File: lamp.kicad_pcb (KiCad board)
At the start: 4 copper layers, 24 x 24 mm, 47 parts, among them J1 Conn_01x01_Female, J2 Conn_01x01_Female, J3 Conn_01x01_Female, J4 Conn_01x01_Female, J5 Conn_01x01_Female, J6 Conn_01x01_Female, J7 Conn_01x01_Female, U1 STM32F030F4P6, U2 LMV321, U3 MIC5205-3.3, U4 TPS54620, U5 LMV321

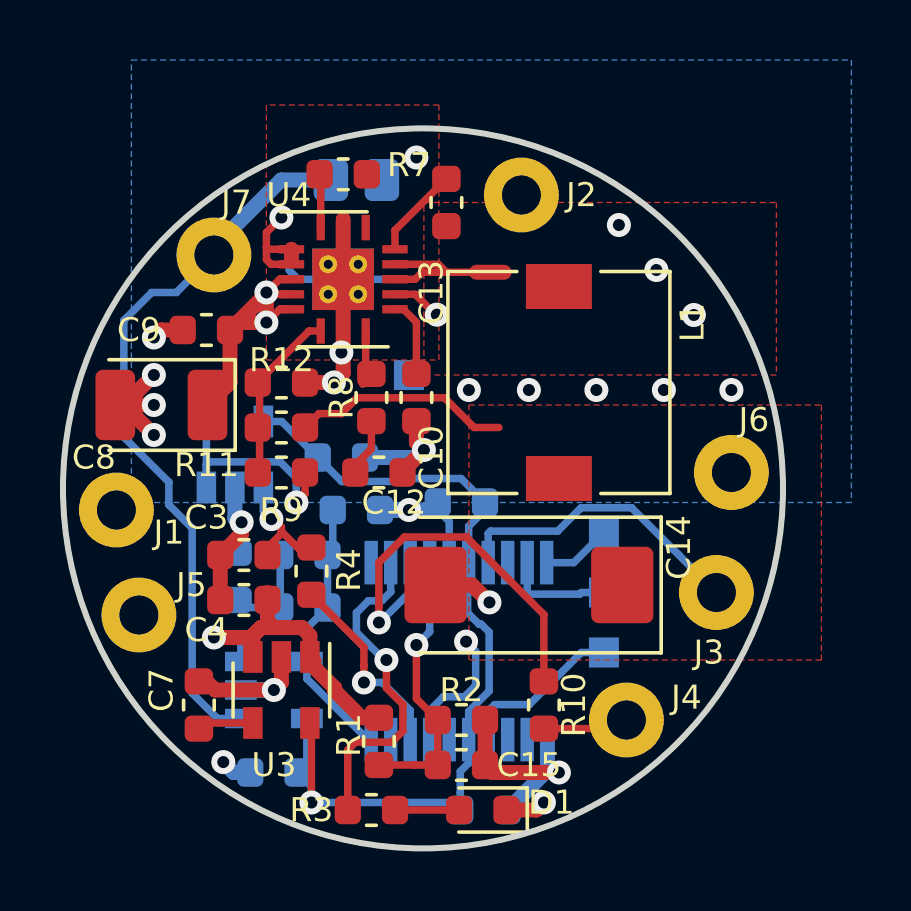
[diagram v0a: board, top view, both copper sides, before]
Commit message: Wibbles
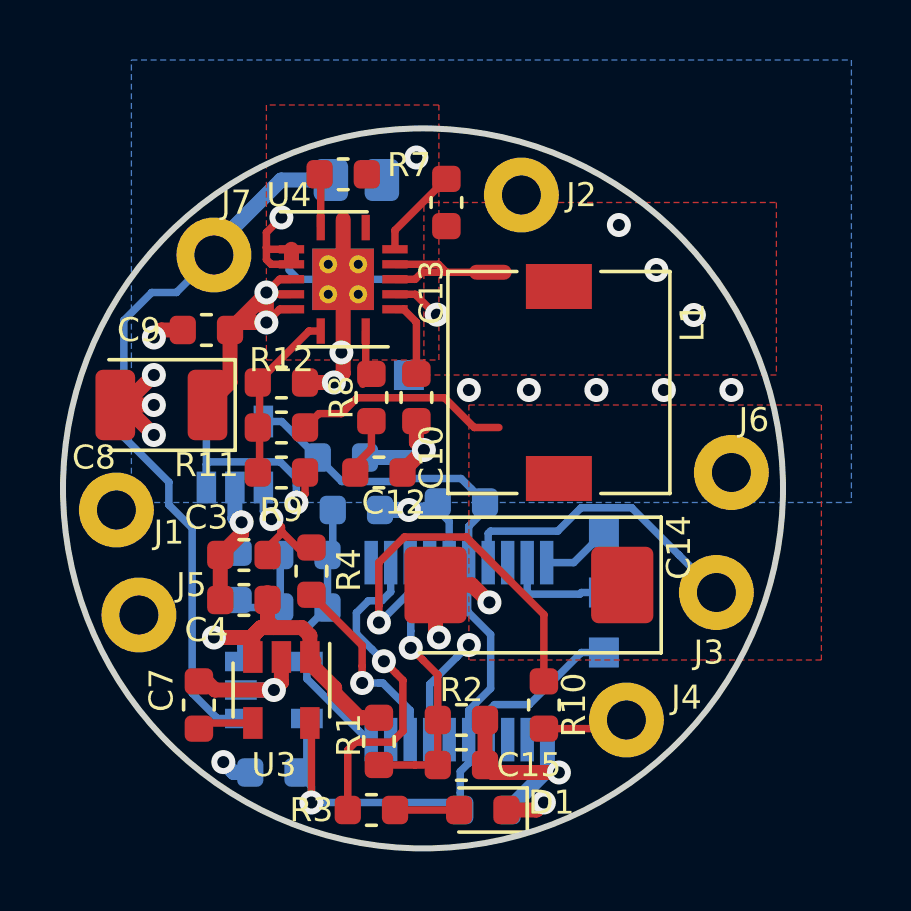
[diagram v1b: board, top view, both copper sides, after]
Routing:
- net GND: track 57.6 -> 59.4 mm, vias 24 -> 25
- net /EN: track 17.4 -> 16.8 mm
